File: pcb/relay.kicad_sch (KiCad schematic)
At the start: 3 parts, among them K3 CRR05-1A, Q3 BSS84

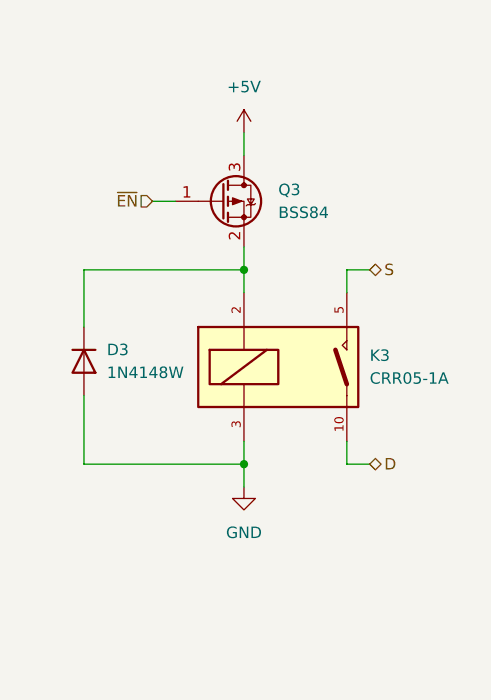
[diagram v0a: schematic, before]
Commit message: chore: many changes checkpoint
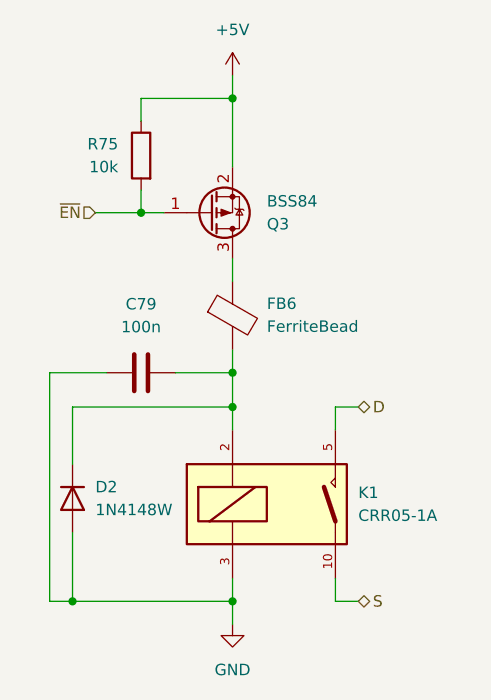
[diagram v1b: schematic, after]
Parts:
- removed D3: 1N4148W, Diode_SMD:D_SOD-123, symbol Diode:1N4148W
- removed K3: CRR05-1A, symbol project_library:CRR05-1A
- added C79: 100n, Capacitor_SMD:C_0603_1608Metric, symbol Device:C
- added D2: 1N4148W, Diode_SMD:D_SOD-123, symbol Diode:1N4148W
- added FB6: FerriteBead, Inductor_SMD:L_0603_1608Metric, symbol Device:FerriteBead
- added K1: CRR05-1A, project_library:CRR05-1A, symbol project_library:CRR05-1A
- added R75: 10k, Resistor_SMD:R_0603_1608Metric, symbol Device:R
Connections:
- net +5V: now also Q3.2 (S), R75.1; no longer Q3.3 (D)
- net D: now also K1.5
- net GND: now also C79.2, D2.2 (A), K1.3
- net S: now also K1.10
- net ~{EN}: now also R75.2
- new net: C79.1, D2.1 (K), FB6.2, K1.2
- new net: FB6.1, Q3.3 (D)
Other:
- moved on the sheet: Q3
